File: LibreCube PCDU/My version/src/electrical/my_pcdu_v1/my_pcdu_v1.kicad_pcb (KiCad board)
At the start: 2 copper layers, 90.2 x 95.9 mm, 0 parts

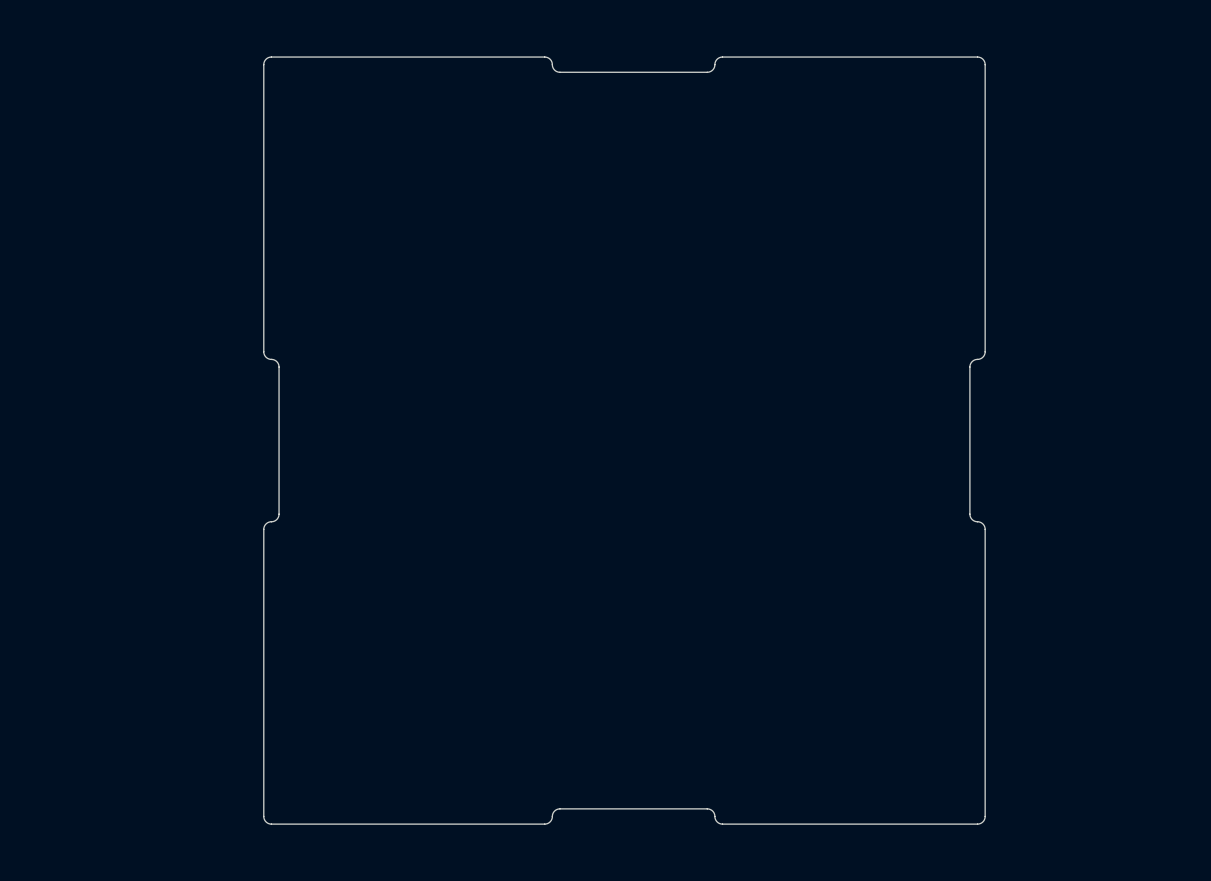
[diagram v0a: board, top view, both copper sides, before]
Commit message: More updates
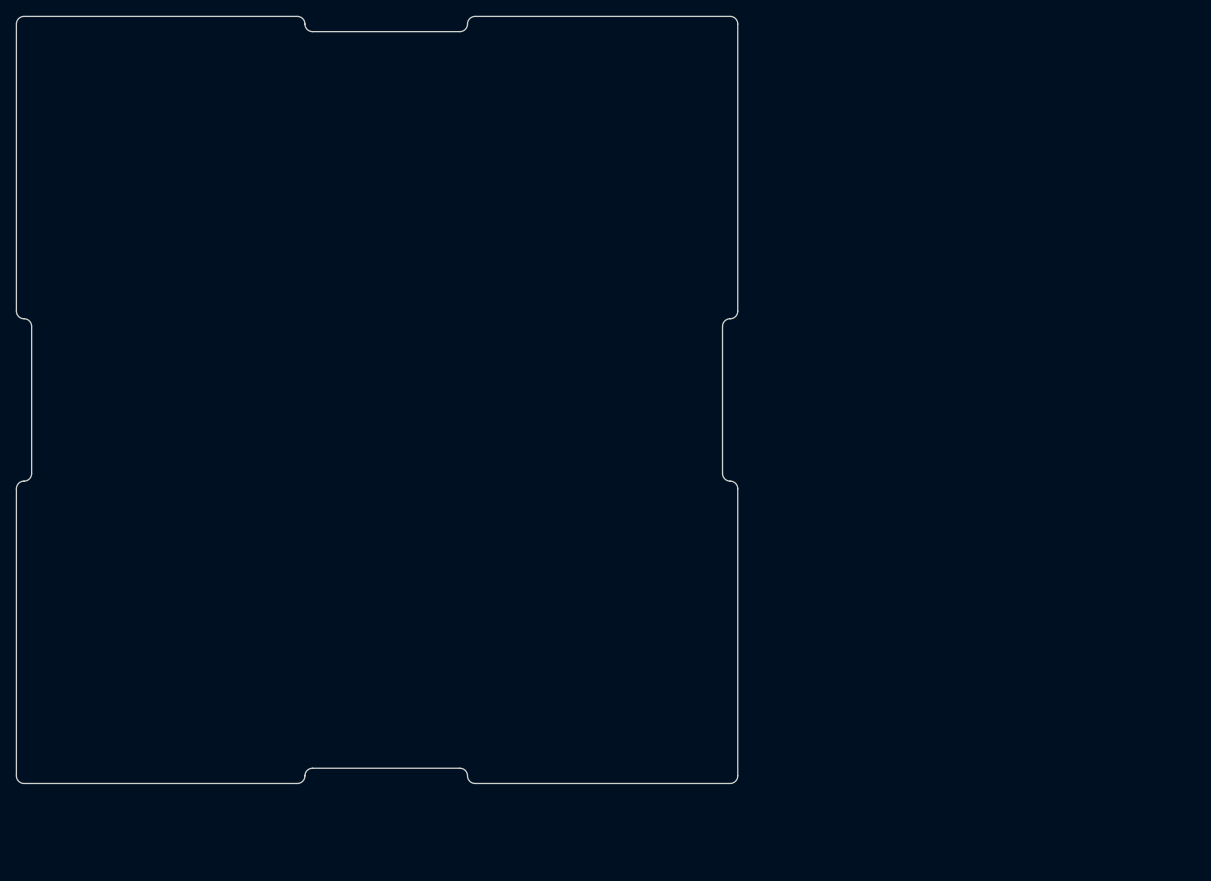
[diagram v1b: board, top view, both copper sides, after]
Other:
- copper layers 2 -> 4

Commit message: Updates
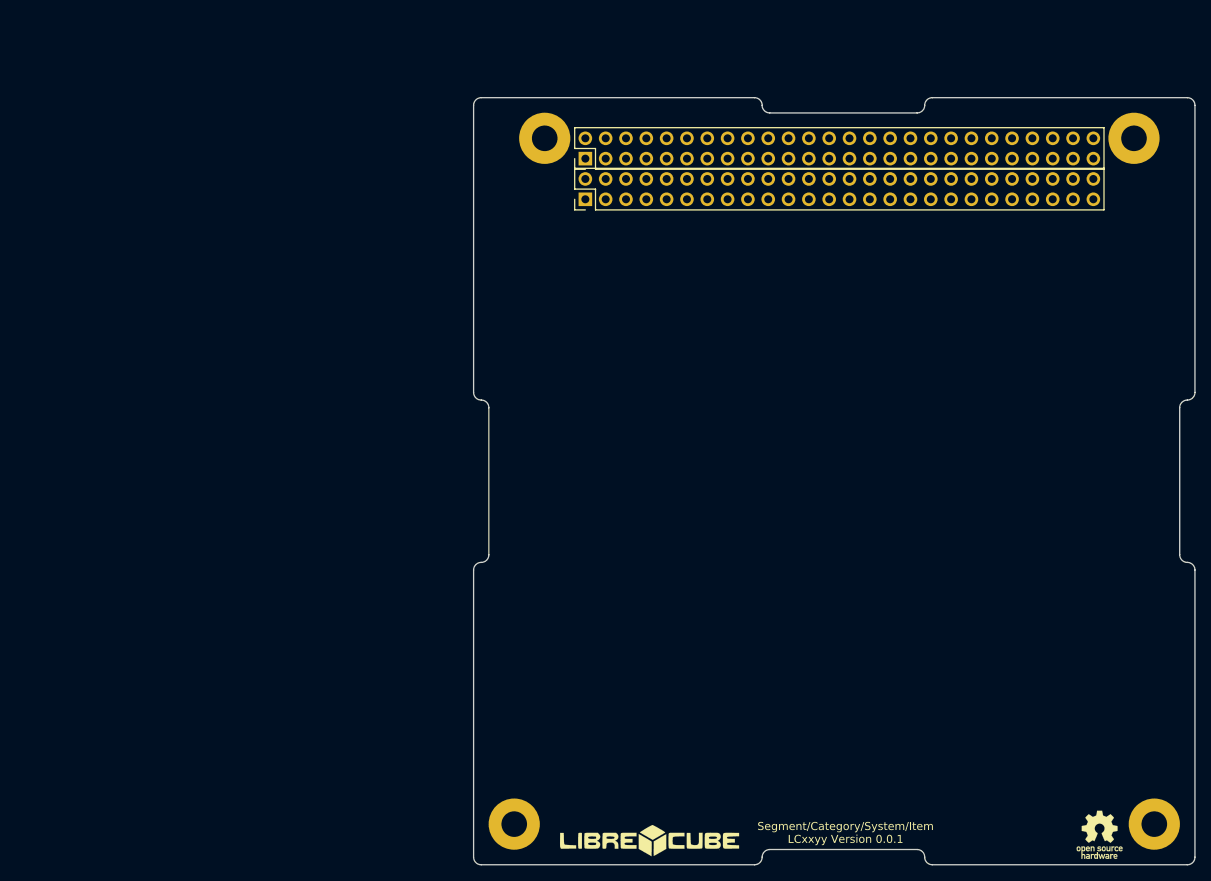
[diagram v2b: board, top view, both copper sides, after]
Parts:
- added G***: LOGO, librecube_pcb_template:LibreCube_logo_22.4mm, F.Cu at (104.5, 134.2)
- added H1: ESQ-126-39-x-D, Connector_PinHeader_2.54mm:PinHeader_2x26_P2.54mm_Vertical, F.Cu at (96.5, 54.0)
- added H2: ESQ-126-39-x-D, Connector_PinHeader_2.54mm:PinHeader_2x26_P2.54mm_Vertical, F.Cu at (96.5, 48.9)
- added M1: MountingHole, MountingHole:MountingHole_3.2mm_M3_Pad, F.Cu at (91.4, 46.4)
- added M2: MountingHole, MountingHole:MountingHole_3.2mm_M3_Pad, F.Cu at (165.1, 46.4)
- added M3: MountingHole, MountingHole:MountingHole_3.2mm_M3_Pad, F.Cu at (167.6, 132.1)
- added M4: MountingHole, MountingHole:MountingHole_3.2mm_M3_Pad, F.Cu at (87.6, 132.1)
- added REF1: Logo_Open_Hardware_Small, Symbol:OSHW-Logo_5.7x6mm_SilkScreen, F.Cu at (160.8, 133.4)
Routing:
- added copper zone on In1.Cu, net /GND
- added copper zone on In2.Cu, net /GND
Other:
- board text added: "Segment/Category/System/Item LCxxyy Version 0.0.1"
